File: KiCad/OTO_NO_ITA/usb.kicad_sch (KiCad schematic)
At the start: 4 parts, among them Q1 STL40DN3LLH5, Q2 STL40DN3LLH5, U3 TCPP03-M20, U4 ECMF2-40A100N6

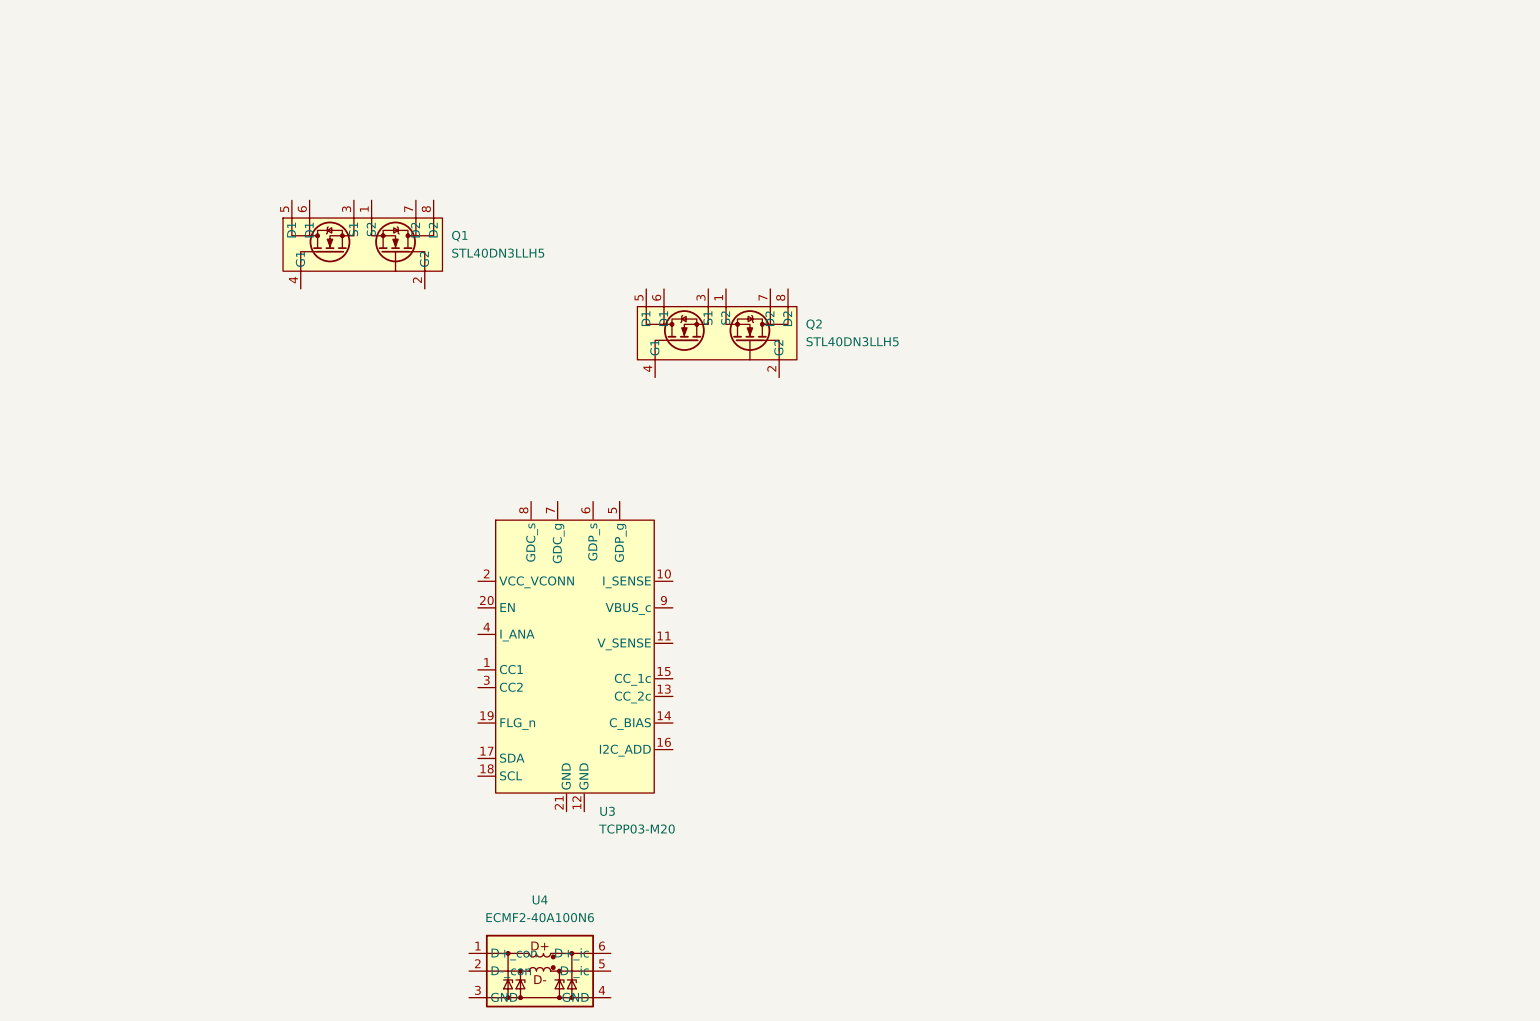
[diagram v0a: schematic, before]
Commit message: Updated schematics.
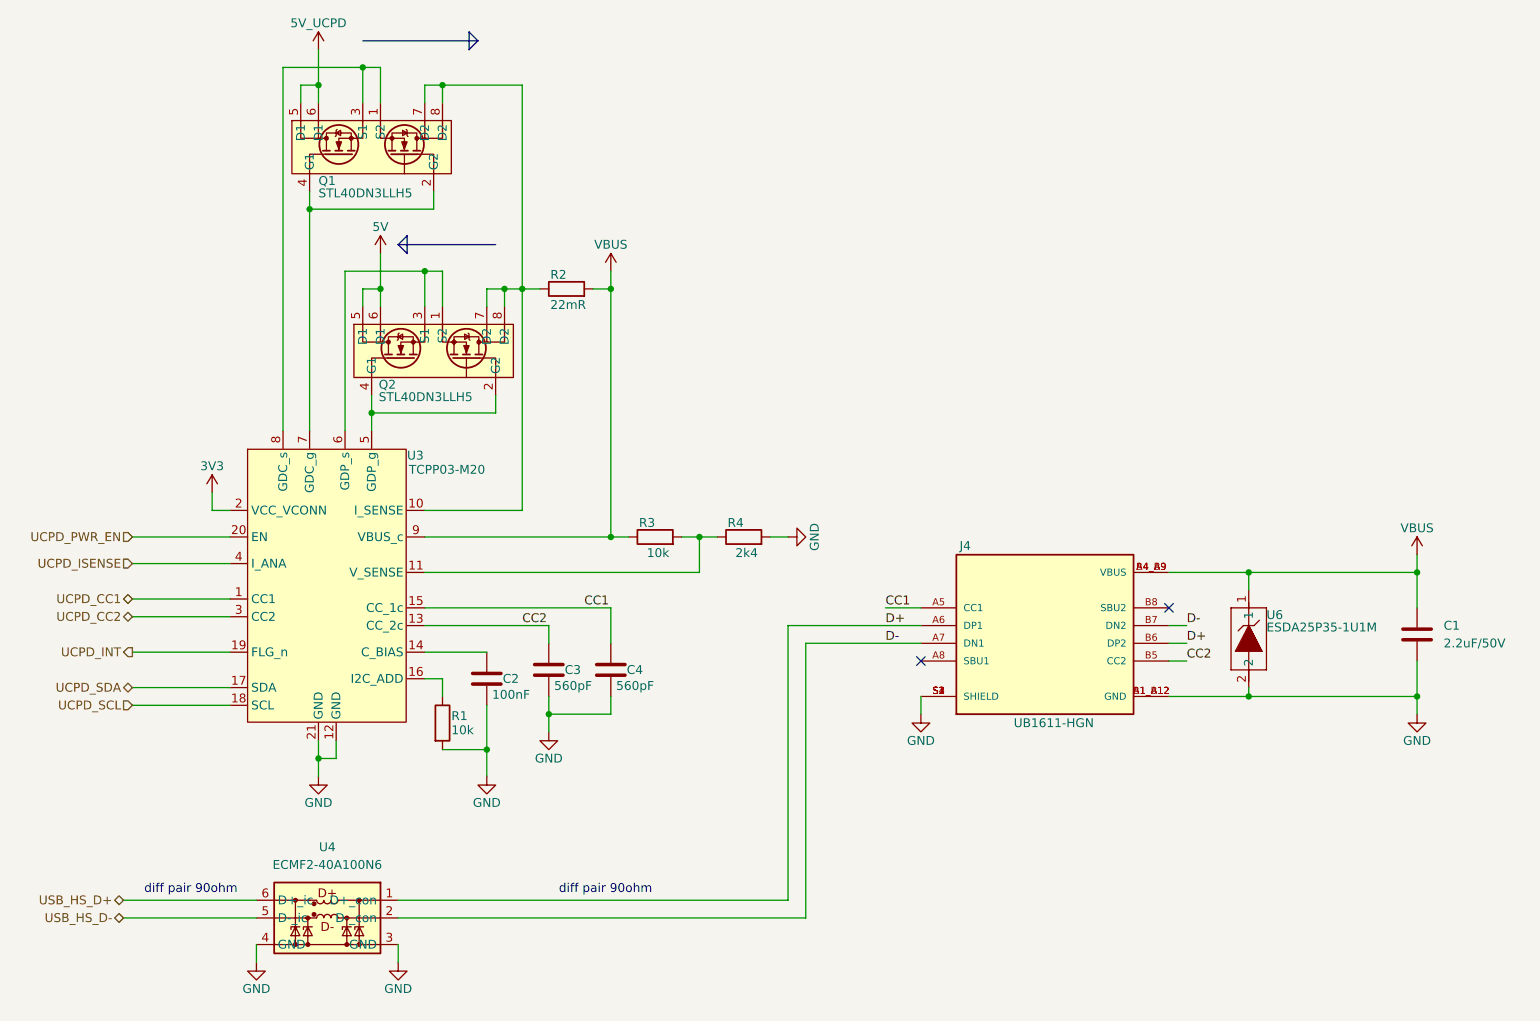
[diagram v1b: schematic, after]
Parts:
- added C1: 2.2uF/50V, symbol Device:C
- added C2: 100nF, symbol Device:C
- added C3, C4: 560pF, symbol Device:C
- added J4: UB1611-HGN, My_Parts:Gangyuan_UB1611-HGN, symbol My_Parts:5077CR-16SMC2-BK-TR
- added R1, R3: 10k, symbol Device:R
- added R2: 22mR, symbol Device:R
- added R4: 2k4, symbol Device:R
- added U6: ESDA25P35-1U1M, symbol My_Parts:ESDA25P35-1U1M
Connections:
- net UCPD_CC1: now reaches U3.1 (CC1)
- net at U3.10 (I_SENSE): now also Q1.7 (D2), Q1.8 (D2), Q2.7 (D2), Q2.8 (D2), R2.1
- net at U3.11 (V_SENSE): now also R3.2, R4.1
- net GND: now reaches U3.12 (GND)
- net GND: now also U3.21 (GND), U4.3 (GND), U4.4 (GND), C1.2, C2.2, C3.2, C4.2, J4.A1_B12 (GND), J4.B1_A12 (GND), J4.S1 (SHIELD), J4.S2 (SHIELD), J4.S3 (SHIELD), J4.S4 (SHIELD), R1.2, R4.2, U6.2
- net CC2: now reaches U3.13 (CC_2c)
- net CC2: now also C3.1, J4.B5 (CC2)
- net at U3.14 (C_BIAS): now also C2.1
- net CC1: now reaches U3.15 (CC_1c)
- net CC1: now also C4.1, J4.A5 (CC1)
- net at U3.16 (I2C_ADD): now also R1.1
- net UCPD_SDA: now reaches U3.17 (SDA)
- net UCPD_SCL: now reaches U3.18 (SCL)
- net UCPD_INT: now reaches U3.19 (FLG_n)
- net 3V3: now reaches U3.2 (VCC_VCONN)
- net UCPD_PWR_EN: now reaches U3.20 (EN)
- net UCPD_CC2: now reaches U3.3 (CC2)
- net UCPD_ISENSE: now reaches U3.4 (I_ANA)
- net at U3.5 (GDP_g): now also Q2.2 (G2), Q2.4 (G1)
- net at U3.6 (GDP_s): now also Q2.1 (S2), Q2.3 (S1)
- net at U3.7 (GDC_g): now also Q1.2 (G2), Q1.4 (G1)
- net at U3.8 (GDC_s): now also Q1.1 (S2), Q1.3 (S1)
- net VBUS: now reaches U3.9 (VBUS_c)
- net VBUS: now also C1.1, J4.A4_B9 (VBUS), J4.B4_A9 (VBUS), R2.2, R3.1, U6.1
- net 5V_UCPD: now reaches Q1.5 (D1)
- net 5V_UCPD: now also Q1.6 (D1)
- net 5V: now reaches Q2.5 (D1)
- net 5V: now also Q2.6 (D1)
- net D+: now reaches U4.1 (D+_con)
- net D+: now also J4.A6 (DP1), J4.B6 (DP2)
- net D-: now reaches U4.2 (D-_con)
- net D-: now also J4.A7 (DN1), J4.B7 (DN2)
- net USB_HS_D-: now reaches U4.5 (D-_ic)
- net USB_HS_D+: now reaches U4.6 (D+_ic)
- no-connect marks 0 -> 2
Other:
- note added: "diff pair 90ohm"
- moved on the sheet: Q1, Q2, U3, U4
